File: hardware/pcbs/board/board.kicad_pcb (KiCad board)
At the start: 2 copper layers, 153.4 x 104.5 mm, 72 parts, among them K00 Key, K01 Key, K02 Key, K03 Key, K10 Key, K11 Key, K12 Key, K13 Key, K20 Key, K21 Key, K22 Key, K23 Key, K30 Key, K31 Key, K32 Key, K33 Key, K40 Key, K41 Key, K42 Key, K43 Key, K50 Key, K51 Key, K52 Key, K53 Key, K60 Key, K61 Key

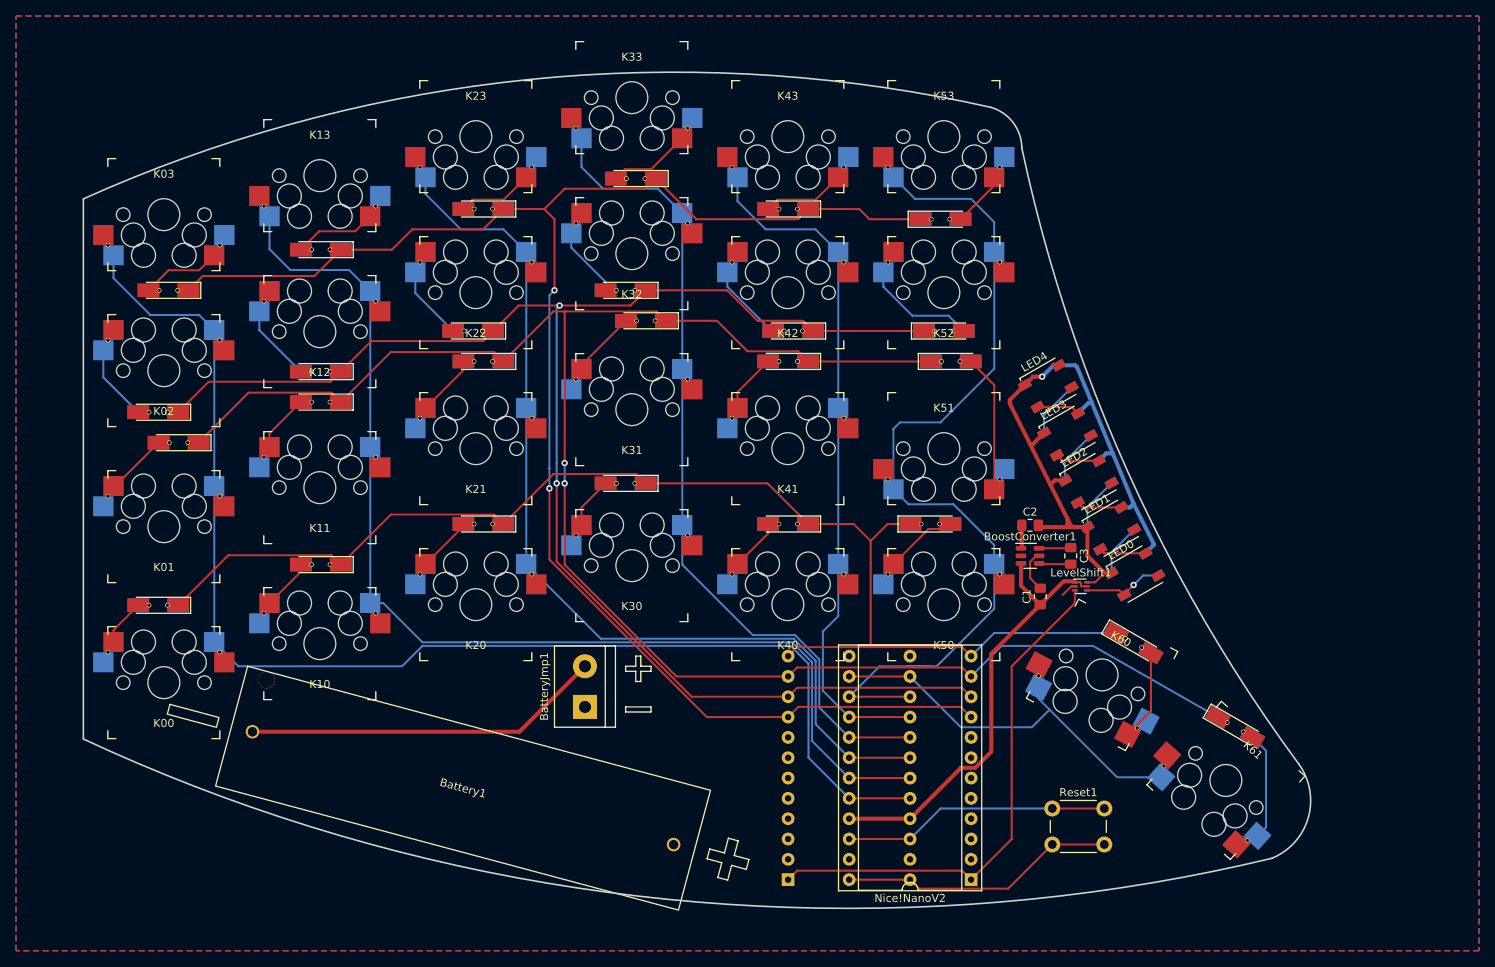
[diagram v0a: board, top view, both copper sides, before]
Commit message: updates to pcb and case
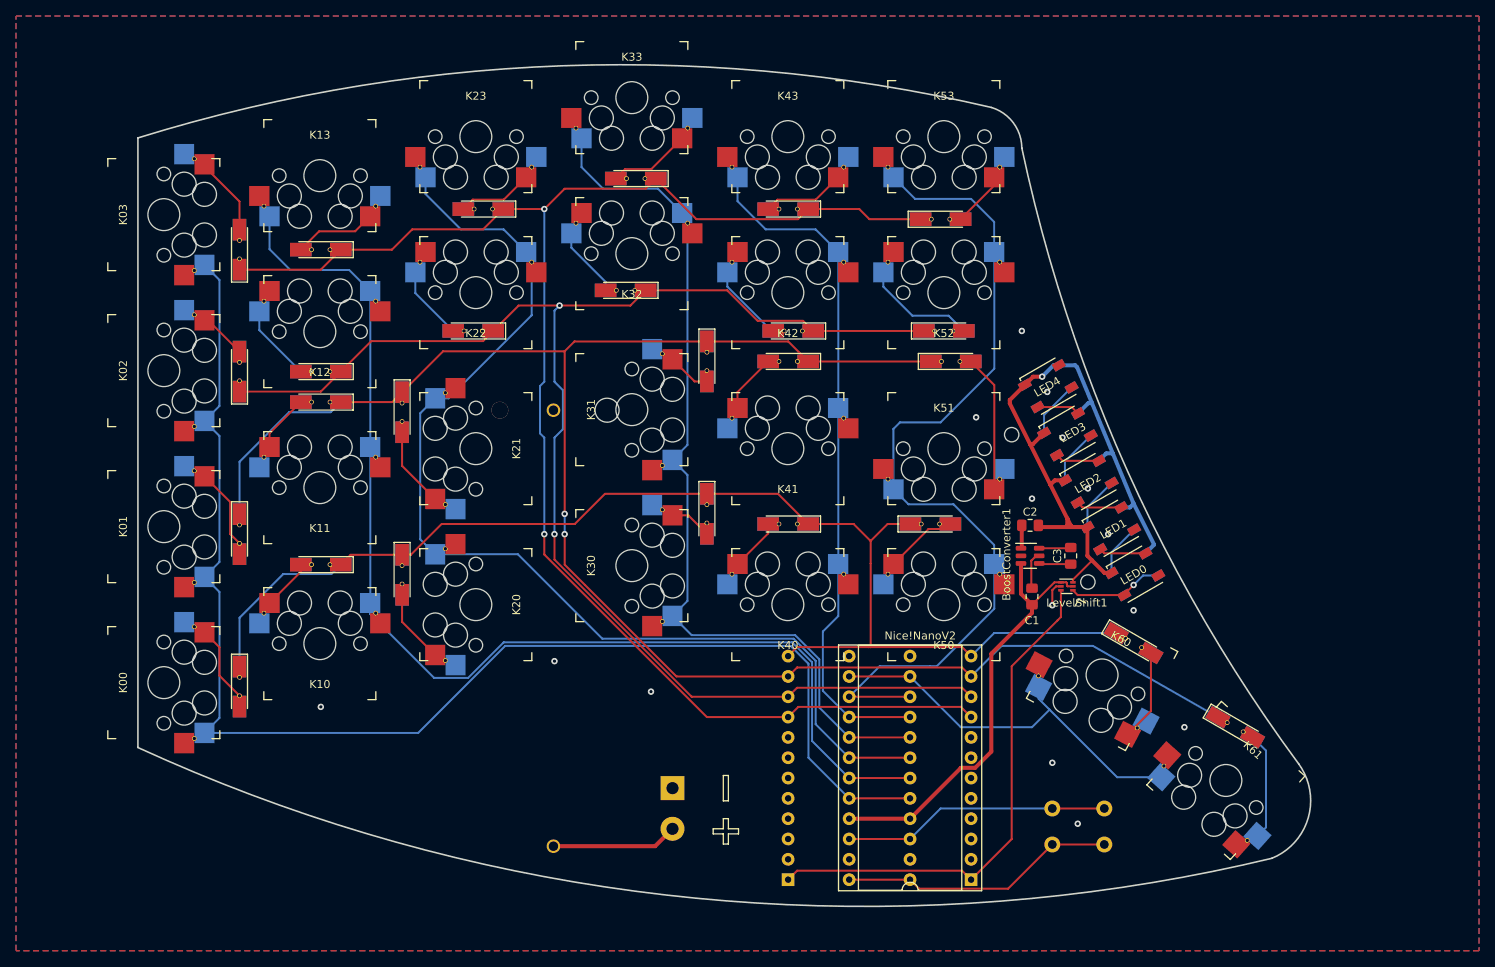
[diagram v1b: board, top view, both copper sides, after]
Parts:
- Battery1, BatteryJmp1, Reset1: moved to B.Cu
- moved Battery1 23.0 mm to (135.8, 112.1), turned to -90 degrees
- moved BatteryJmp1 14.9 mm to (150.6, 132.1), turned to -90 degrees
- moved D00 14.4 mm to (96.5, 119.4), turned to -90 degrees
- moved D01 13.7 mm to (96.5, 100.3), turned to -90 degrees
- moved D21 12.0 mm to (116.8, 85.1), turned to -90 degrees
- moved D20 12.0 mm to (116.8, 105.4), turned to -90 degrees
- moved D02 11.4 mm to (96.5, 80.0), turned to 90 degrees
- moved D30 10.9 mm to (154.9, 97.8), turned to -90 degrees
- moved D03 10.2 mm to (96.5, 64.8), turned to 90 degrees
- moved D31 9.16 mm to (154.9, 78.7), turned to -90 degrees
- moved Reset1 6.50 mm to (204.6, 134.6), turned to 180 degrees
- moved LevelShift1 1.75 mm to (199.9, 106.8)
- moved C1 1.03 mm to (195.6, 108.1)
- turned K00 to -90 degrees
- turned K01 to -90 degrees
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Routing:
- net Net-(Battery1-Pad1): track 45.0 -> 15.8 mm
- net Col2: track 119.4 -> 136.3 mm
- net Col0: track 161.2 -> 170.6 mm
- net Row1: track 226.9 -> 219.2 mm
- net Row2: track 193.5 -> 185.9 mm
- net Col3: track 103.5 -> 111.0 mm
- net Row3: track 207.0 -> 199.5 mm
- net Row0: track 161.0 -> 156.1 mm
- net Col1: track 140.2 -> 144.7 mm
- net Net-(D00-Pad2): track 5.87 -> 9.74 mm
- net Net-(D02-Pad2): track 9.55 -> 6.00 mm
- net Net-(D31-Pad2): track 8.32 -> 5.45 mm
- net Col5: track 113.1 -> 110.3 mm
- net Net-(D01-Pad2): track 7.87 -> 10.2 mm
- net Net-(D20-Pad2): track 6.96 -> 9.23 mm
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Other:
- board size 153.4 x 104.5 mm -> 146.6 x 105.2 mm
- board text added: "Light Barrier"
